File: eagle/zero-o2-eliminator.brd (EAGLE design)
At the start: 12.4 x 54.6 mm, 8 parts, among them IC1 L7805, U1 TINY85-20-DIP

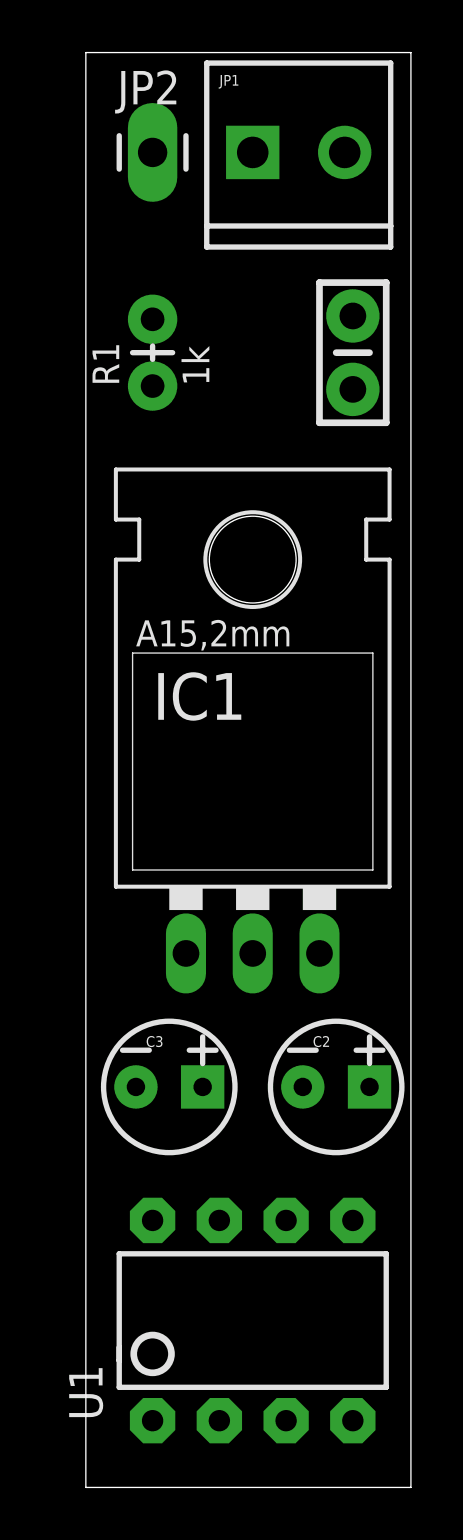
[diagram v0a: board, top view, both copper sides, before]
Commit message: latest
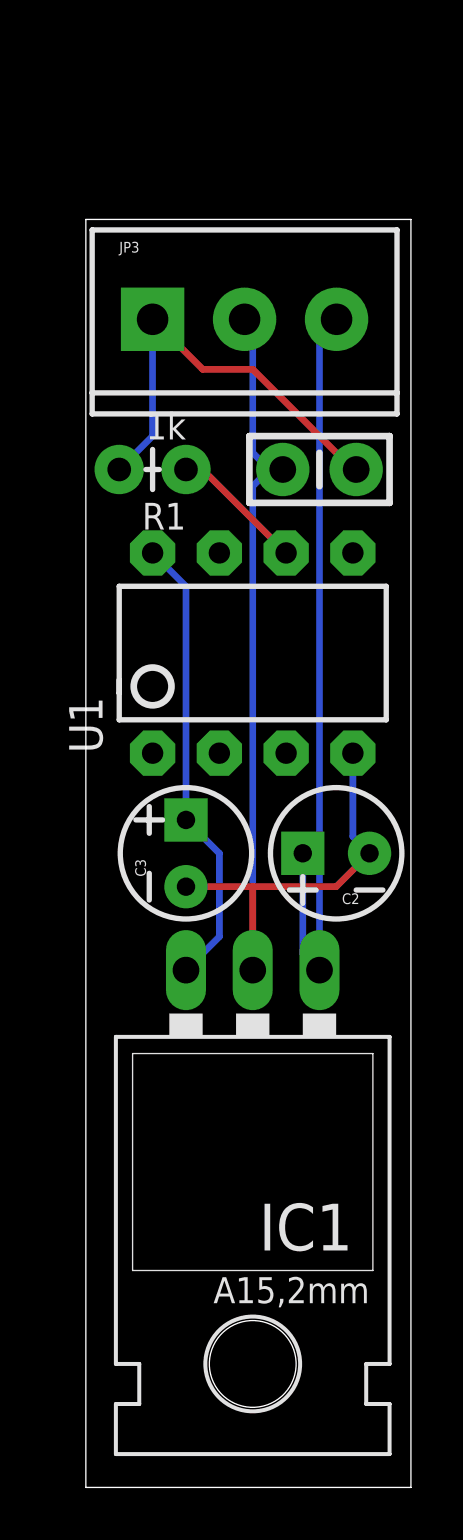
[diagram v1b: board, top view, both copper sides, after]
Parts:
- removed JP1: M023.5MM, SparkFun-Connectors:SCREWTERMINAL-3.5MM-2
- removed JP2: SIG, SparkFun-Connectors:1X01_LONGPAD
- added JP3: (no value), SparkFun-Connectors:SCREWTERMINAL-3.5MM-3
- moved U1 25.4 mm to (6.35, 31.8)
- moved C3 8.91 mm to (3.81, 24.1), turned to 90 degrees
- moved C2 8.89 mm to (9.53, 24.1), turned to 180 degrees
- moved IC1 8.25 mm to (6.35, 15.9), turned to 180 degrees
- moved C1 4.62 mm to (8.89, 38.7), turned to 180 degrees
- moved R1 3.42 mm to (3.81, 38.7), turned to 180 degrees
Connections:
- removed net 3.3V: C1.2, C2.2, C3.2, IC1.GND, JP1.1, U1.4
- removed net N$2: C1.1, JP2.1, R1.P$2
- removed net N$3: C2.1, IC1.IN, JP1.2
- new net 12V: C2.1, IC1.IN, JP3.3
- new net GND: C1.2, C2.2, C3.2, IC1.GND, JP3.2, U1.4
- new net OUT: C1.1, JP3.1, R1.P$2
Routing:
- net GND: track 0.00 -> 40.9 mm
- net 12V: track 0.00 -> 29.8 mm
- net N$4: track 0.00 -> 17.5 mm
- net OUT: track 0.00 -> 16.4 mm
- net N$1: track 0.00 -> 5.13 mm
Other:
- board size 12.4 x 54.6 mm -> 12.4 x 48.2 mm
- board text added: "Micah Pearlman www.zeroengineering.io"
- board text added: "Zero O2 Eliminator"
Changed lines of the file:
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@@
 <plain>
 <wire x1="0" y1="0" x2="12.37" y2="0" width="0" layer="20"/>
-<wire x1="12.37" y1="0" x2="12.37" y2="54.6" width="0" layer="20"/>
-<wire x1="12.37" y1="54.6" x2="0" y2="54.6" width="0" layer="20"/>
-<wire x1="0" y1="54.6" x2="0" y2="0" width="0" layer="20"/>
+<wire x1="12.37" y1="0" x2="12.37" y2="48.25" width="0" layer="20"/>
+<wire x1="12.37" y1="48.25" x2="0" y2="48.25" width="0" layer="20"/>
+<wire x1="0" y1="48.25" x2="0" y2="0" width="0" layer="20"/>
+<text x="10.16" y="1.27" size="1.778" layer="122" font="fixed" rot="MR90">Zero O2 Eliminator</text>
+<text x="1.27" y="1.27" size="1.4224" layer="122" font="fixed" rot="MR90">Micah Pearlman
+www.zeroengineering.io</text>
 </plain>
 <attributes>
@@
 <param name="RoutingGrid" value="50mil"/>
 <param name="AutoGrid" value="1"/>
-<param name="Efforts" value="0"/>
+<param name="Efforts" value="2"/>
 <param name="TopRouterVariant" value="1"/>
 <param name="tpViaShape" value="round"/>
@@
 </autorouter>
 <elements>
-<element name="C1" library="SparkFun-Capacitors" package="CAP-PTH-SMALL-KIT" value="0.1uF" x="10.16" y="43.18" rot="R90">
-<attribute name="PROD_ID" value="CAP-08370" x="10.16" y="43.18" size="1.778" layer="27" rot="R90" display="off"/>
-</element>
-<element name="C2" library="SparkFun-Capacitors" package="CPOL-RADIAL-10UF-25V-KIT" value="100uF" x="9.525" y="15.24">
-<attribute name="PROD_ID" value="CAP-08440" x="9.525" y="15.24" size="1.778" layer="27" display="off"/>
-</element>
-<element name="C3" library="SparkFun-Capacitors" package="CPOL-RADIAL-10UF-25V-KIT" value="10uF" x="3.175" y="15.24">
-<attribute name="PROD_ID" value="CAP-08440" x="3.175" y="15.24" size="1.778" layer="27" display="off"/>
-</element>
-<element name="IC1" library="SparkFun-PowerIC" package="78XXL" value="L7805" x="6.35" y="24.13"/>
-<element name="JP1" library="SparkFun-Connectors" package="SCREWTERMINAL-3.5MM-2" value="M023.5MM" x="6.35" y="50.8"/>
-<element name="JP2" library="SparkFun-Connectors" package="1X01_LONGPAD" value="SIG" x="2.54" y="50.8"/>
-<element name="R1" library="SparkFun-Resistors" package="AXIAL-0.1EZ" value="1k" x="2.54" y="41.91" rot="R90">
-<attribute name="PROD_ID" value="RES-08380" x="2.54" y="41.91" size="1.778" layer="27" rot="R90" display="off"/>
-</element>
-<element name="U1" library="SparkFun-DigitalIC" package="DIP08" value="TINY85-20-DIP" x="6.35" y="6.35">
-<attribute name="PROD_ID" value="IC-09445" x="6.35" y="6.35" size="1.778" layer="27" display="off"/>
-</element>
+<element name="C1" library="SparkFun-Capacitors" package="CAP-PTH-SMALL-KIT" value="0.1uF" x="8.89" y="38.735" rot="R180">
+<attribute name="PROD_ID" value="CAP-08370" x="8.89" y="38.735" size="1.778" layer="27" rot="R180" display="off"/>
+</element>
+<element name="C2" library="SparkFun-Capacitors" package="CPOL-RADIAL-10UF-25V-KIT" value="100uF" x="9.525" y="24.13" rot="R180">
+<attribute name="PROD_ID" value="CAP-08440" x="9.525" y="24.13" size="1.778" layer="27" rot="R180" display="off"/>
+</element>
+<element name="C3" library="SparkFun-Capacitors" package="CPOL-RADIAL-10UF-25V-KIT" value="10uF" x="3.81" y="24.13" rot="R90">
+<attribute name="PROD_ID" value="CAP-08440" x="3.81" y="24.13" size="1.778" layer="27" rot="R90" display="off"/>
+</element>
+<element name="IC1" library="SparkFun-PowerIC" package="78XXL" value="L7805" x="6.35" y="15.875" rot="R180"/>
+<element name="R1" library="SparkFun-Resistors" package="AXIAL-0.1EZ" value="1k" x="3.81" y="38.735" rot="R180">
+<attribute name="PROD_ID" value="RES-08380" x="3.81" y="38.735" size="1.778" layer="27" rot="R180" display="off"/>
+</element>
+<element name="U1" library="SparkFun-DigitalIC" package="DIP08" value="TINY85-20-DIP" x="6.35" y="31.75">
+<attribute name="PROD_ID" value="IC-09445" x="6.35" y="31.75" size="1.778" layer="27" display="off"/>
+</element>
+<element name="JP3" library="SparkFun-Connectors" package="SCREWTERMINAL-3.5MM-3" value="" x="2.54" y="44.45"/>
 </elements>
 <signals>
-<signal name="3.3V">
+<signal name="GND">
 <contactref element="U1" pad="4"/>
 <contactref element="C1" pad="2"/>
@@
 <contactref element="C3" pad="2"/>
 <contactref element="IC1" pad="GND"/>
-<contactref element="JP1" pad="1"/>
-<wire x1="6.35" y1="50.8" x2="10.16" y2="44.577" width="0" layer="19" extent="1-1"/>
-<wire x1="8.255" y1="15.24" x2="6.35" y2="50.8" width="0" layer="19" extent="1-1"/>
-<wire x1="1.905" y1="15.24" x2="8.255" y2="15.24" width="0" layer="19" extent="1-1"/>
-<wire x1="10.16" y1="2.54" x2="6.35" y2="50.8" width="0" layer="19" extent="1-1"/>
-<wire x1="6.35" y1="20.32" x2="10.16" y2="2.54" width="0" layer="19" extent="1-1"/>
+<contactref element="JP3" pad="2"/>
+<wire x1="6.35" y1="39.37" x2="6.985" y2="38.735" width="0.254" layer="16"/>
+<wire x1="6.35" y1="44.45" x2="6.35" y2="39.37" width="0.254" layer="16"/>
+<wire x1="6.35" y1="44.45" x2="6.04" y2="44.45" width="0.254" layer="16"/>
+<wire x1="10.16" y1="24.765" x2="10.795" y2="24.13" width="0.254" layer="16"/>
+<wire x1="10.16" y1="27.94" x2="10.16" y2="24.765" width="0.254" layer="16"/>
+<wire x1="6.35" y1="22.86" x2="6.35" y2="19.685" width="0.254" layer="1"/>
+<wire x1="3.81" y1="22.86" x2="6.35" y2="22.86" width="0.254" layer="1"/>
+<wire x1="9.525" y1="22.86" x2="10.795" y2="24.13" width="0.254" layer="1"/>
+<wire x1="6.35" y1="22.86" x2="9.525" y2="22.86" width="0.254" layer="1"/>
+<wire x1="6.35" y1="38.1" x2="6.985" y2="38.735" width="0.254" layer="16"/>
+<wire x1="6.35" y1="19.685" x2="6.35" y2="38.1" width="0.254" layer="16"/>
+<wire x1="6.985" y1="38.735" x2="7.493" y2="38.735" width="0.254" layer="16"/>
 </signal>
 <signal name="N$1">
 <contactref element="U1" pad="6"/>
 <contactref element="R1" pad="P$1"/>
-<wire x1="2.54" y1="41.91" x2="7.62" y2="10.16" width="0" layer="19" extent="1-1"/>
-</signal>
-<signal name="N$2">
+<wire x1="4.445" y1="38.735" x2="7.62" y2="35.56" width="0.254" layer="1"/>
+<wire x1="3.81" y1="38.735" x2="4.445" y2="38.735" width="0.254" layer="1"/>
+</signal>
+<signal name="OUT">
 <contactref element="R1" pad="P$2"/>
 <contactref element="C1" pad="1"/>
-<contactref element="JP2" pad="1"/>
-<wire x1="2.54" y1="44.45" x2="10.16" y2="41.783" width="0" layer="19" extent="1-1"/>
-<wire x1="2.54" y1="50.8" x2="2.54" y2="44.45" width="0" layer="19" extent="1-1"/>
-</signal>
-<signal name="N$3">
+<contactref element="JP3" pad="1"/>
+<wire x1="2.54" y1="40.005" x2="1.27" y2="38.735" width="0.254" layer="16"/>
+<wire x1="2.54" y1="44.45" x2="2.54" y2="40.005" width="0.254" layer="16"/>
+<wire x1="6.35" y1="42.545" x2="10.16" y2="38.735" width="0.254" layer="1"/>
+<wire x1="4.445" y1="42.545" x2="6.35" y2="42.545" width="0.254" layer="1"/>
+<wire x1="2.54" y1="44.45" x2="4.445" y2="42.545" width="0.254" layer="1"/>
+<wire x1="10.16" y1="38.735" x2="10.287" y2="38.735" width="0.254" layer="1"/>
+</signal>
+<signal name="12V">
 <contactref element="IC1" pad="IN"/>
 <contactref element="C2" pad="1"/>
-<contactref element="JP1" pad="2"/>
-<wire x1="10.795" y1="15.24" x2="9.85" y2="50.8" width="0" layer="19" extent="1-1"/>
-<wire x1="3.81" y1="20.32" x2="9.85" y2="50.8" width="0" layer="19" extent="1-1"/>
+<contactref element="JP3" pad="3"/>
+<wire x1="8.255" y1="20.32" x2="8.89" y2="19.685" width="0.254" layer="16"/>
+<wire x1="8.255" y1="24.13" x2="8.255" y2="20.32" width="0.254" layer="16"/>
+<wire x1="8.89" y1="43.815" x2="9.525" y2="44.45" width="0.254" layer="16"/>
+<wire x1="8.89" y1="19.685" x2="8.89" y2="43.815" width="0.254" layer="16"/>
+<wire x1="9.525" y1="44.45" x2="9.54" y2="44.45" width="0.254" layer="16"/>
 </signal>
 <signal name="N$4">
@@
 <contactref element="C3" pad="1"/>
 <contactref element="U1" pad="8"/>
-<wire x1="2.54" y1="10.16" x2="8.89" y2="20.32" width="0" layer="19" extent="1-1"/>
-<wire x1="4.445" y1="15.24" x2="2.54" y2="10.16" width="0" layer="19" extent="1-1"/>
+<wire x1="5.08" y1="20.955" x2="3.81" y2="19.685" width="0.254" layer="16"/>
+<wire x1="5.08" y1="24.13" x2="5.08" y2="20.955" width="0.254" layer="16"/>
+<wire x1="3.81" y1="25.4" x2="5.08" y2="24.13" width="0.254" layer="16"/>
+<wire x1="3.81" y1="34.29" x2="2.54" y2="35.56" width="0.254" layer="16"/>
+<wire x1="3.81" y1="25.4" x2="3.81" y2="34.29" width="0.254" layer="16"/>
 </signal>
 </signals>
 </board>
 </drawing>
+<compatibility>
+<note version="6.3" minversion="6.2.2" severity="warning">
+Since Version 6.2.2 text objects can contain more than one line,
+which will not be processed correctly with this version.
+</note>
+</compatibility>
 </eagle>
